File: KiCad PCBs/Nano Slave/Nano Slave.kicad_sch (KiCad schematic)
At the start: 50 parts, among them J1 Screw_Terminal_01x02, J10 AVR-ISP-6, J11 Conn_01x06_Female, J12 Screw_Terminal_01x02, J13 Screw_Terminal_01x02, J14 Screw_Terminal_01x02, J15 Screw_Terminal_01x02, J16 Screw_Terminal_01x02, J2 Screw_Terminal_01x02, J3 Screw_Terminal_01x02, J4 Screw_Terminal_01x02, J5 Screw_Terminal_01x02, J6 Screw_Terminal_01x02, J7 Screw_Terminal_01x02, J8 Screw_Terminal_01x02, J9 Screw_Terminal_01x02, SW1 SW_DIP_x02, SW2 SW_DIP_x02, SW3 SW_MEC_5E, U1 ATmega328P-AU, U2 MAX487ESA+T, U3 ULN2003A, U5 AMS1117-5.0, Y1 Crystal_GND24

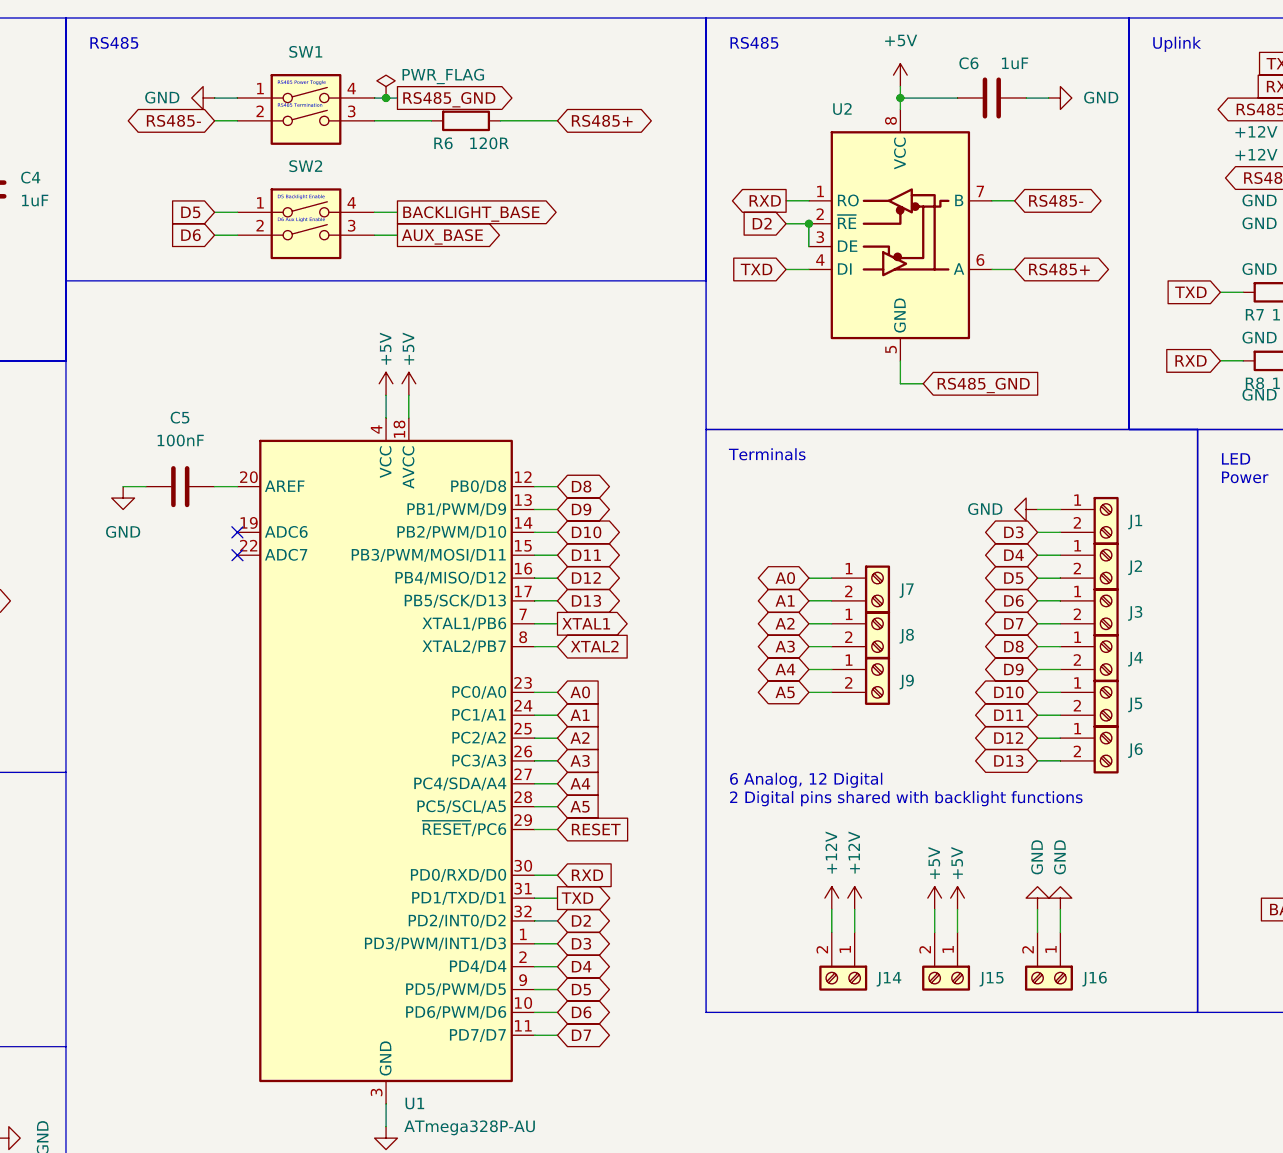
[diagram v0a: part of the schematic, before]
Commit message: Nano Slave Rev 2
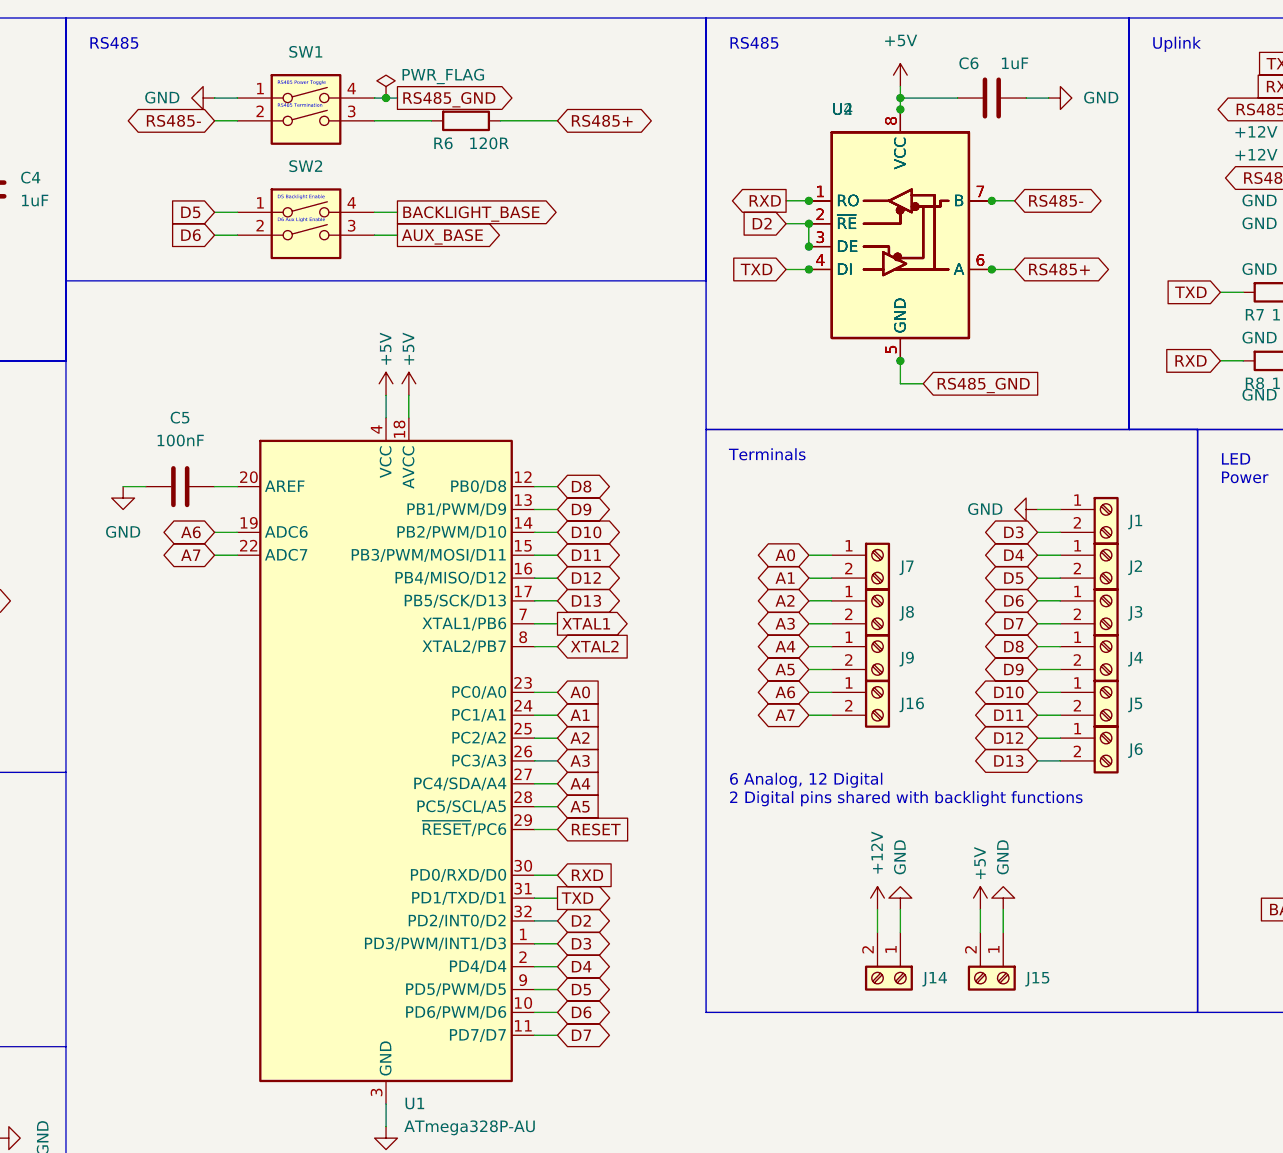
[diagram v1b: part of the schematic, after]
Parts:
- added U4: MAX487CPA+, Package_DIP:DIP-8_W7.62mm, symbol A10:MAX487
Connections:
- net +12V: no longer J14.1 (Pin_1)
- net +5V: now also U4.8 (VCC); no longer J15.1 (Pin_1)
- net D2: now also U4.2 (~{RE}), U4.3 (DE)
- net GND: now also J14.1 (Pin_1), J15.1 (Pin_1); no longer J16.1 (Pin_1), J16.2 (Pin_2)
- net RS485+: now also U4.6 (A)
- net RS485-: now also U4.7 (B)
- net RS485_GND: now also U4.5 (GND)
- net RXD: now also U4.1 (RO)
- net TXD: now also U4.4 (DI)
- net A6: now reaches U1.19 (ADC6)
- net A6: now also J16.1 (Pin_1)
- net A7: now reaches U1.22 (ADC7)
- net A7: now also J16.2 (Pin_2)
- no-connect marks 8 -> 6
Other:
- moved on the sheet: J14, J15, J16, J7, J8, J9
